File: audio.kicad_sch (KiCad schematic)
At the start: 50 parts, among them J11 Gain Control, J12 Gain Control, J4 NCJ6FA-H-0, J5 NCJ6FA-H-0, Q2 MMBT3906, Q3 FFB3904, Q4 MMBT3906, Q5 FFB3904, U11 LM2903, U5 THAT1246, U6 THAT1246, U9 OPA1656ID

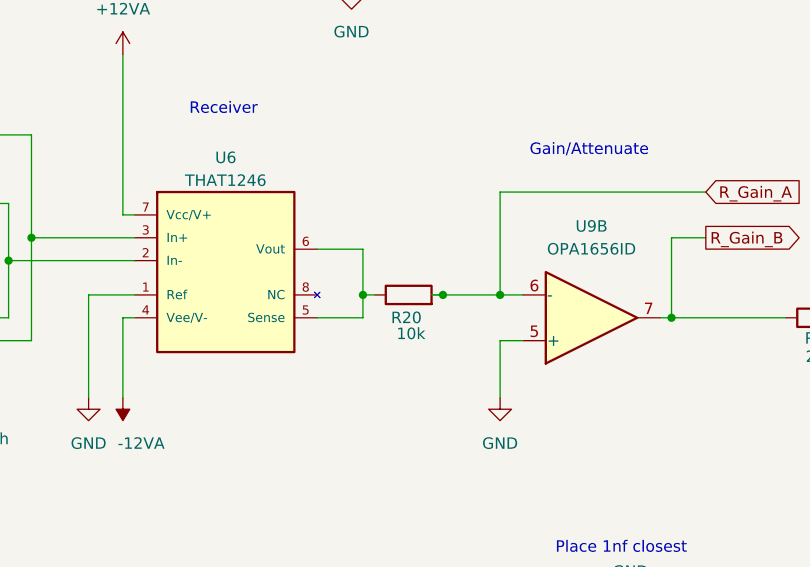
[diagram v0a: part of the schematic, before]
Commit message: output design update
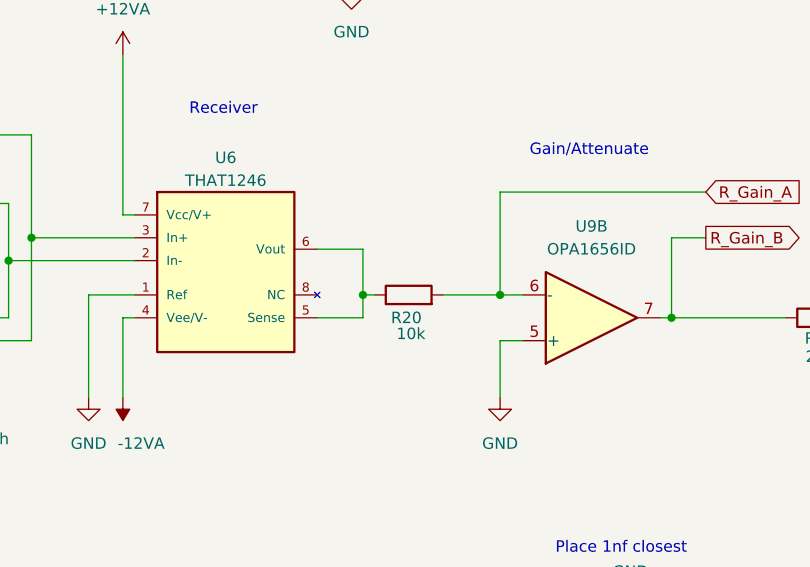
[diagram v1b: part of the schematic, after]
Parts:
- added unit 2 of U11
- added unit 1 of U11
- added unit 2 of U9
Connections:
- net AUDIO_IN_L: now also U11.3 (+); no longer U11.3 (+)
- net AUDIO_IN_R: now also U11.5 (+); no longer U11.5 (+)
- net GND: now also U9.5 (+); no longer U9.5 (+)
- net L_Clip_Led: now also U11.1; no longer U11.1
- net R_Clip_Led: now also U11.7; no longer U11.7
- net R_Gain_A: now also U9.6 (-); no longer U9.6 (-)
- net R_Gain_B: now also U9.7; no longer U9.7
- net at RV2.2: now also U11.6 (-); no longer U11.6 (-)
- net at RV1.2: now also U11.2 (-); no longer U11.2 (-)
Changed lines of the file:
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@@
 	)
 	(junction
-		(at 82.55 125.73)
-		(diameter 0)
-		(color 0 0 0 0)
-	)
-	(junction
 		(at 76.2 180.34)
 		(diameter 0)
@@
 	)
 	(junction
-		(at 91.44 125.73)
+		(at 82.55 125.73)
 		(diameter 0)
 		(color 0 0 0 0)
@@
 	(wire
 		(pts
-			(xy 82.55 125.73) (xy 82.55 120.65)
-		)
-		(stroke
-			(width 0)
-			(type default)
-		)
-	)
-	(wire
-		(pts
 			(xy 142.24 48.26) (xy 142.24 53.34)
 		)
@@
 	(wire
 		(pts
+			(xy 83.82 125.73) (xy 82.55 125.73)
+		)
+		(stroke
+			(width 0)
+			(type default)
+		)
+	)
+	(wire
+		(pts
 			(xy 176.53 111.76) (xy 179.07 111.76)
 		)
@@
 	(wire
 		(pts
-			(xy 82.55 128.27) (xy 82.55 125.73)
+			(xy 82.55 120.65) (xy 82.55 125.73)
 		)
 		(stroke
@@
 	(wire
 		(pts
-			(xy 82.55 125.73) (xy 83.82 125.73)
-		)
-		(stroke
-			(width 0)
-			(type default)
-		)
-	)
-	(wire
-		(pts
 			(xy 55.88 128.27) (xy 57.15 128.27)
 		)
@@
 	(wire
 		(pts
-			(xy 90.17 125.73) (xy 91.44 125.73)
-		)
-		(stroke
-			(width 0)
-			(type default)
-		)
-	)
-	(wire
-		(pts
 			(xy 55.88 116.84) (xy 55.88 99.06)
 		)
@@
 	(wire
 		(pts
+			(xy 82.55 125.73) (xy 82.55 128.27)
+		)
+		(stroke
+			(width 0)
+			(type default)
+		)
+	)
+	(wire
+		(pts
 			(xy 88.9 90.17) (xy 88.9 85.09)
 		)
@@
 			)
 		)
-		(property "Description" "Potentiometer"
+		(property "Description" "Potentiometer - Audio Taper"
 			(at 207.01 144.78 0)
 			(effects
@@
 			)
 		)
-		(property "Description" "Potentiometer"
+		(property "Description" "Potentiometer - Audio Taper"
 			(at 184.15 144.78 0)
 			(effects
